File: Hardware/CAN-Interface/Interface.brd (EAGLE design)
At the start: 99.6 x 99.8 mm, 56 parts, among them J1 34912-8020, J2 34912-8020, J4 632722110112, J5 OBDII-FEMALEFEMALE, Q1 6.5A/20V/35mΩ, Q2 5.8A/30V/35mΩ, Q3 6.5A/20V/35mΩ, Q4 5.8A/30V/35mΩ

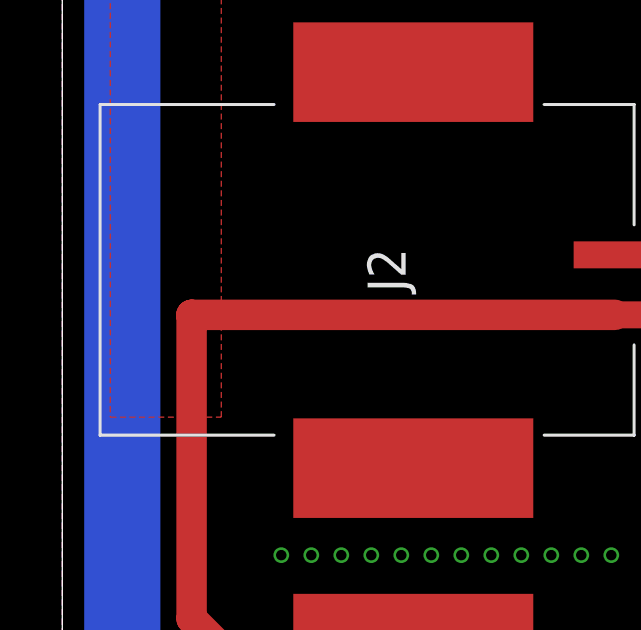
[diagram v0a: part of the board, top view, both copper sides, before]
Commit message: final board prep for manufacture
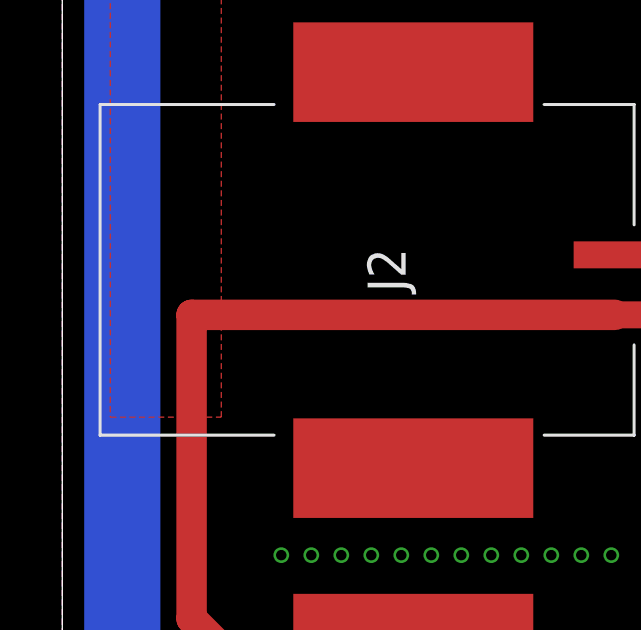
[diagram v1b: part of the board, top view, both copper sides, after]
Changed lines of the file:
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@@
 </polygon>
 <wire x1="18.42" y1="66.41" x2="4.31" y2="66.41" width="1.016" layer="1"/>
-<wire x1="4.31" y1="66.41" x2="4.3" y2="66.4" width="1.016" layer="1"/>
 <wire x1="18.42" y1="47.36" x2="17.505" y2="48.275" width="1.016" layer="1"/>
 <wire x1="17.505" y1="48.275" x2="12.316975" y2="48.275" width="1.016" layer="1"/>
